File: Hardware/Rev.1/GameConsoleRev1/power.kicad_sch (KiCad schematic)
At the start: 0 parts

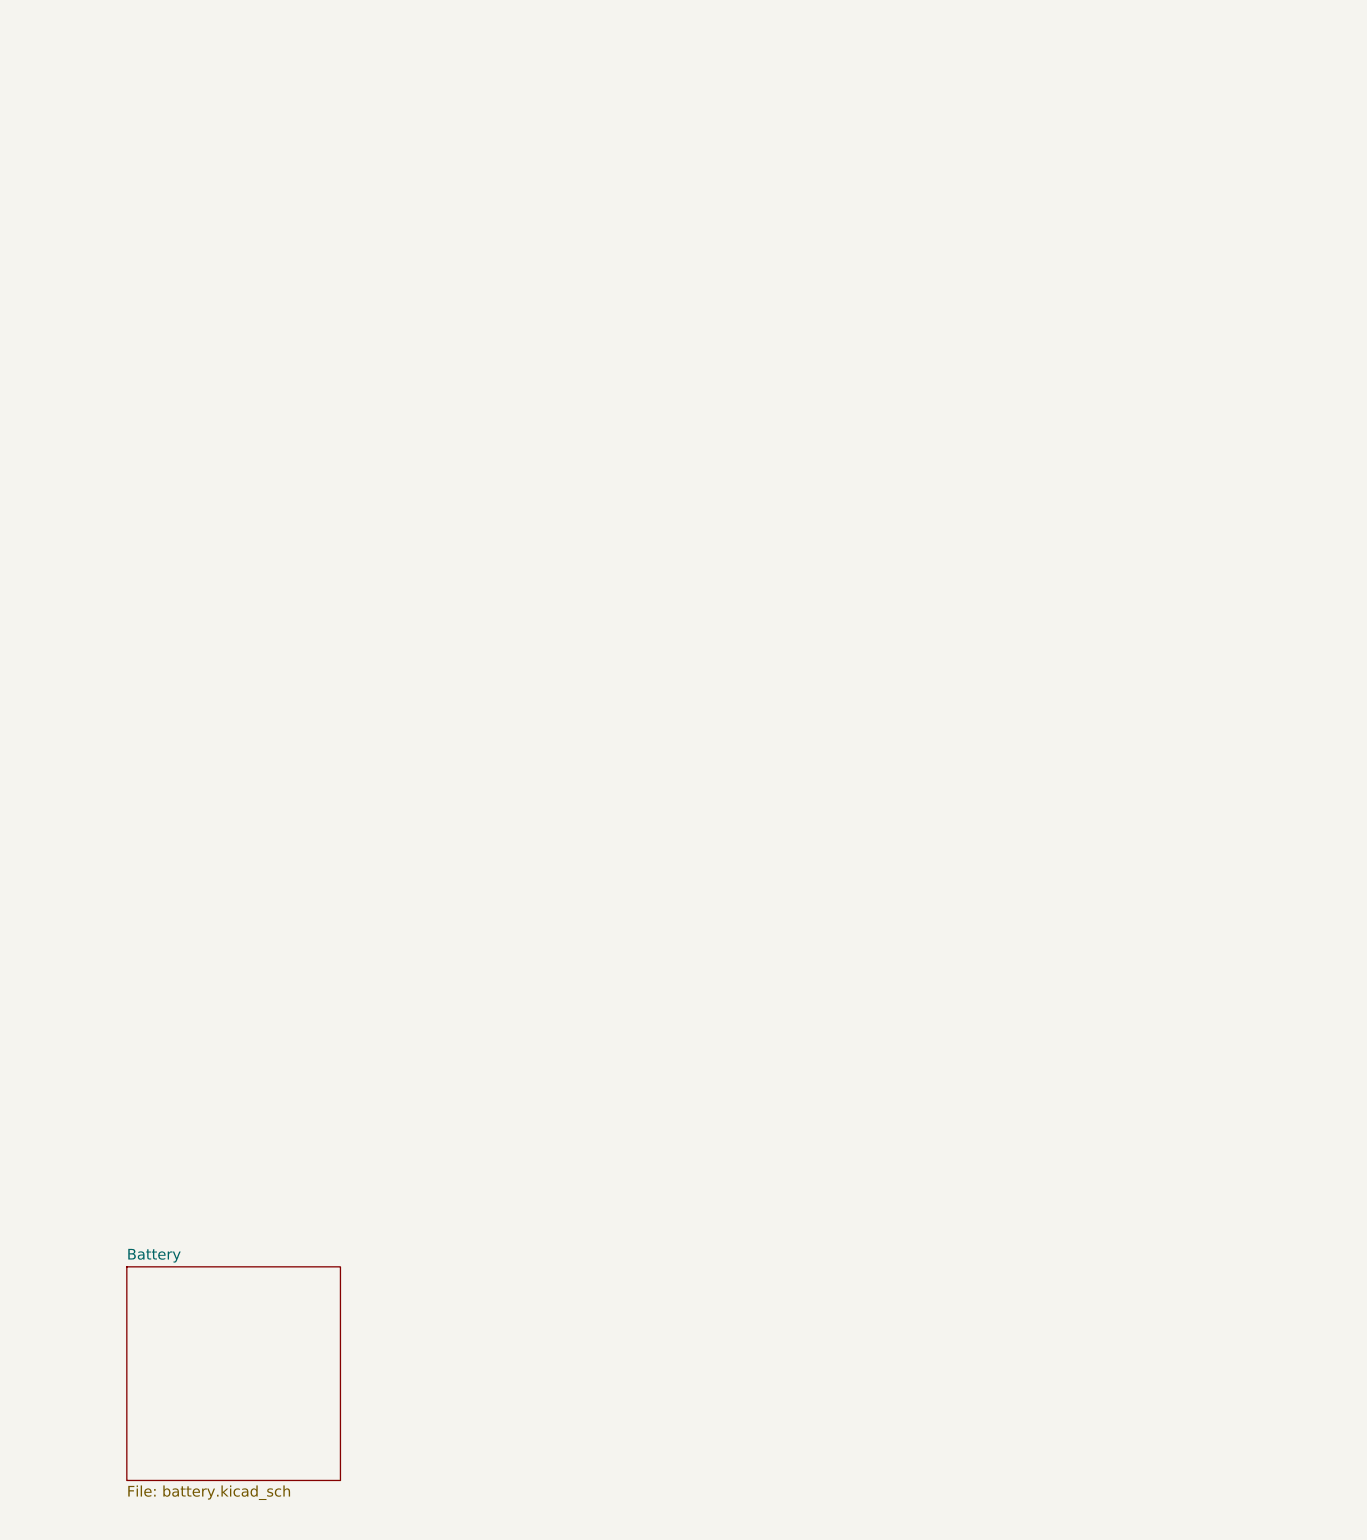
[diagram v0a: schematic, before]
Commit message: Added sprites
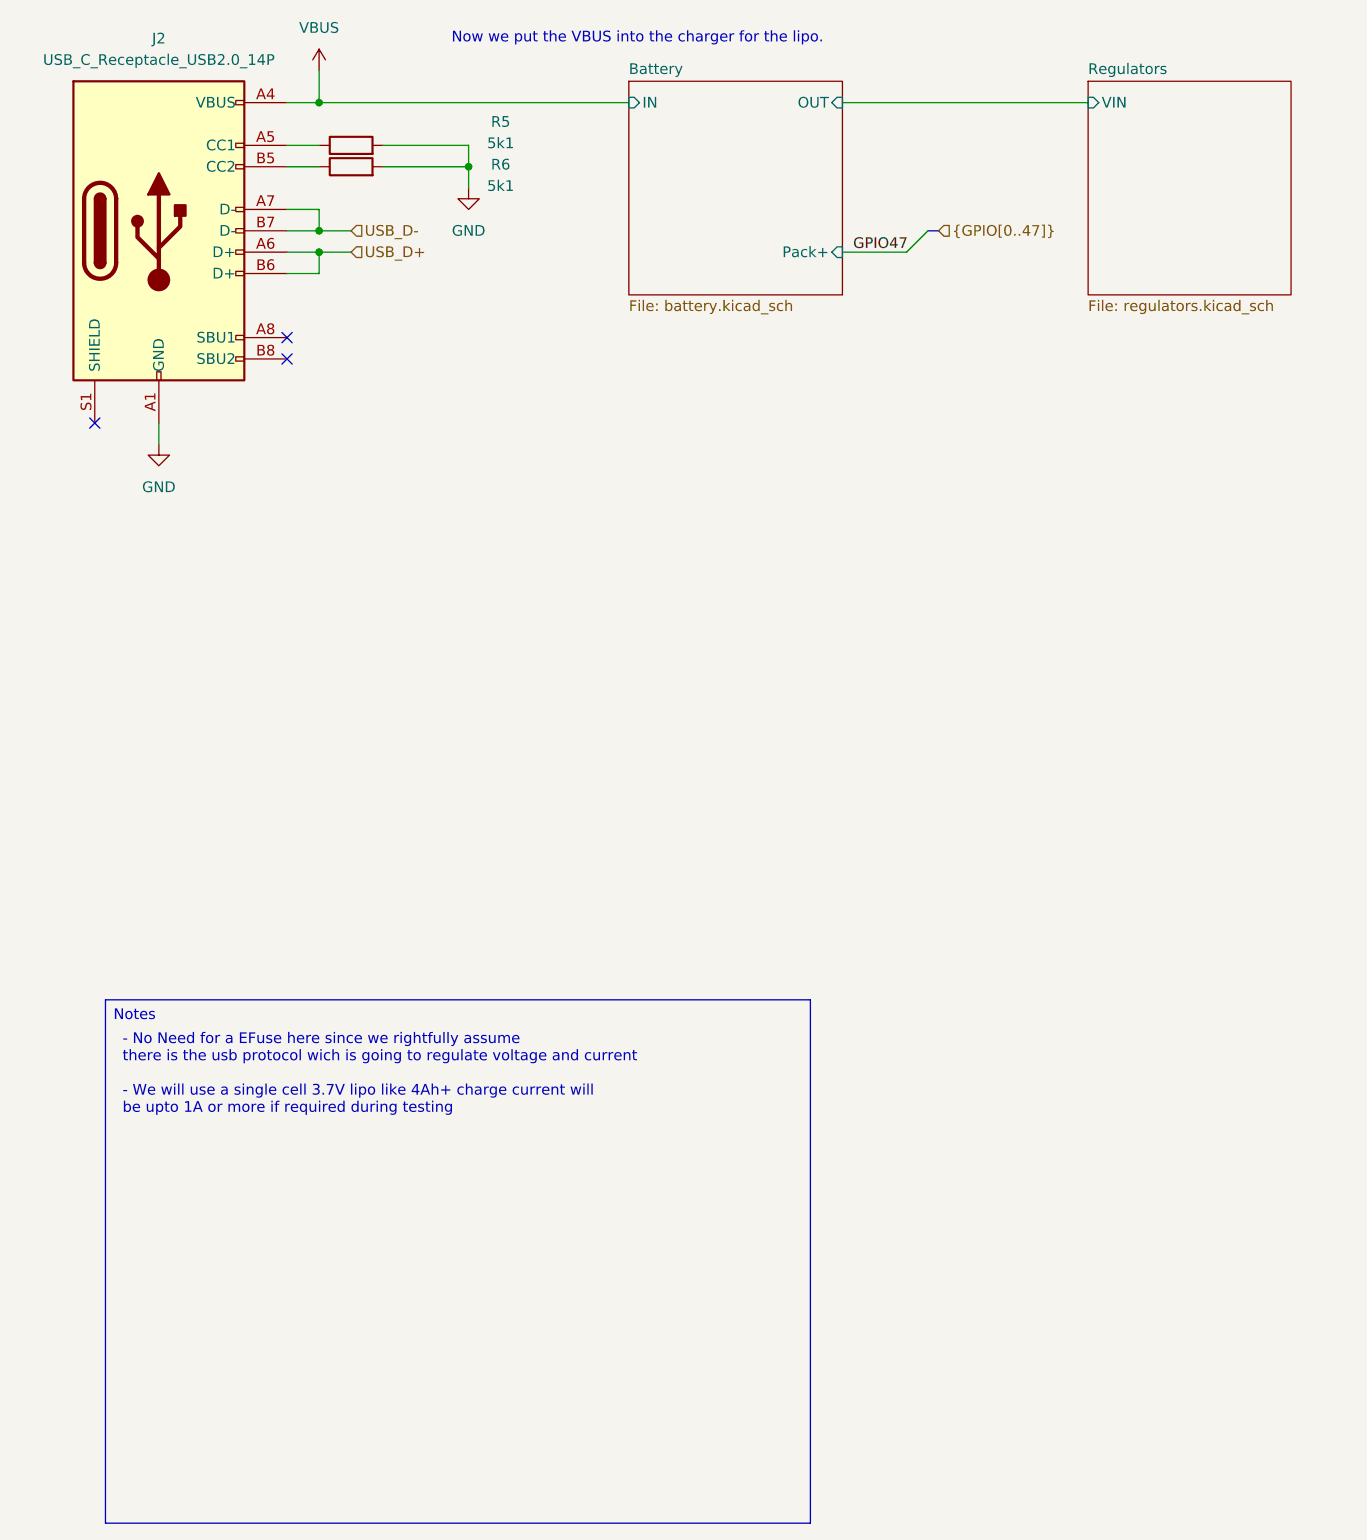
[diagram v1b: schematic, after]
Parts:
- added J2: USB_C_Receptacle_USB2.0_14P, Connector_USB:USB_C_Receptacle_G-Switch_GT-USB-7010ASV, symbol Connector:USB_C_Receptacle_USB2.0_16P
- added R5, R6: 5k1, Resistor_SMD:R_0402_1005Metric, symbol Device:R
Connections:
- new net: J2.A5 (CC1), R5.1
- new net: J2.B5 (CC2), R6.1
- new net GND: J2.A1 (GND), J2.A12 (GND), J2.B1 (GND), J2.B12 (GND), R5.2, R6.2
- new net USB_D+: J2.A6 (D+), J2.B6 (D+)
- new net USB_D-: J2.A7 (D-), J2.B7 (D-)
- new net VBUS: J2.A4 (VBUS), J2.A9 (VBUS), J2.B4 (VBUS), J2.B9 (VBUS)
- no-connect marks 0 -> 3
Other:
- added sheet Regulators (regulators.kicad_sch)
- sheet Battery ports: added IN, OUT, Pack+; removed none
- note added: "- No Need for a EFuse here since we rightfully assume there is the usb protocol wich is going to regulate voltage and current - We will use a single cell 3.7V lipo like 4Ah+ charge current will be upto 1A or more if required during testing"
- note added: "Now we put the VBUS into the charger for the lipo."
